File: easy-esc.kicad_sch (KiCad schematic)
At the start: 43 parts, among them J101 USB_C_Receptacle_USB2.0, J102 BLDC, J103 POWER, SW101 BOOT, SW102 RESET, SW103 EN, U101 TMC6300, U102 XC6206, U103 W25Q128JVS, U104 RP2040, Y101 12MHz

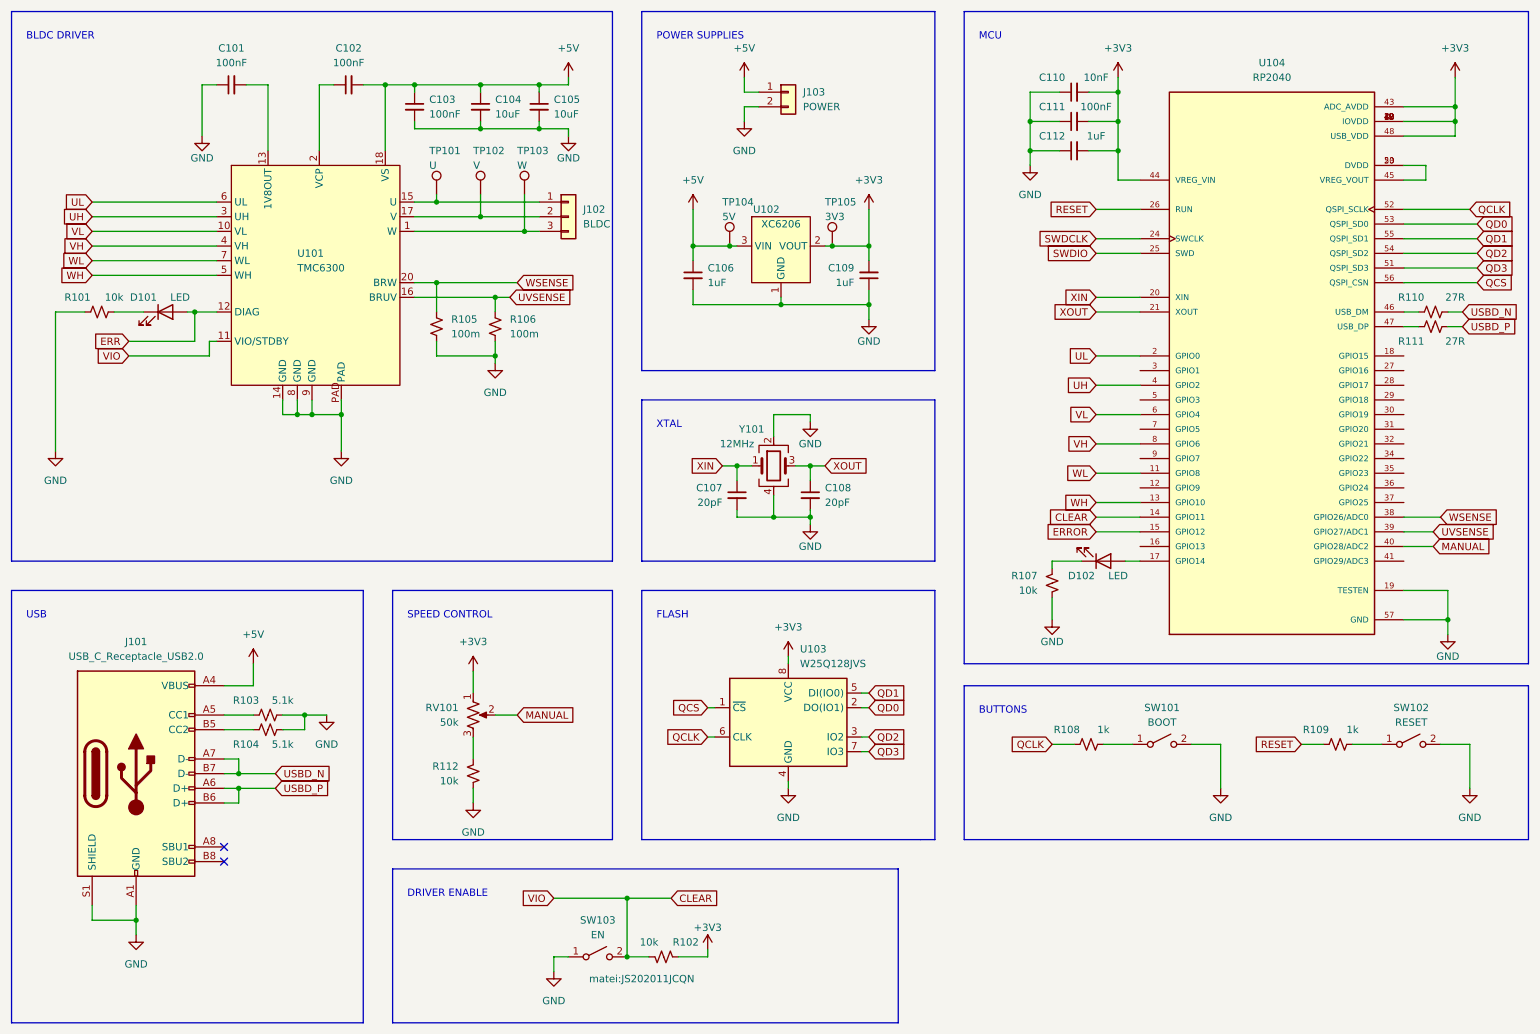
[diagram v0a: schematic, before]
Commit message: finalize fab files
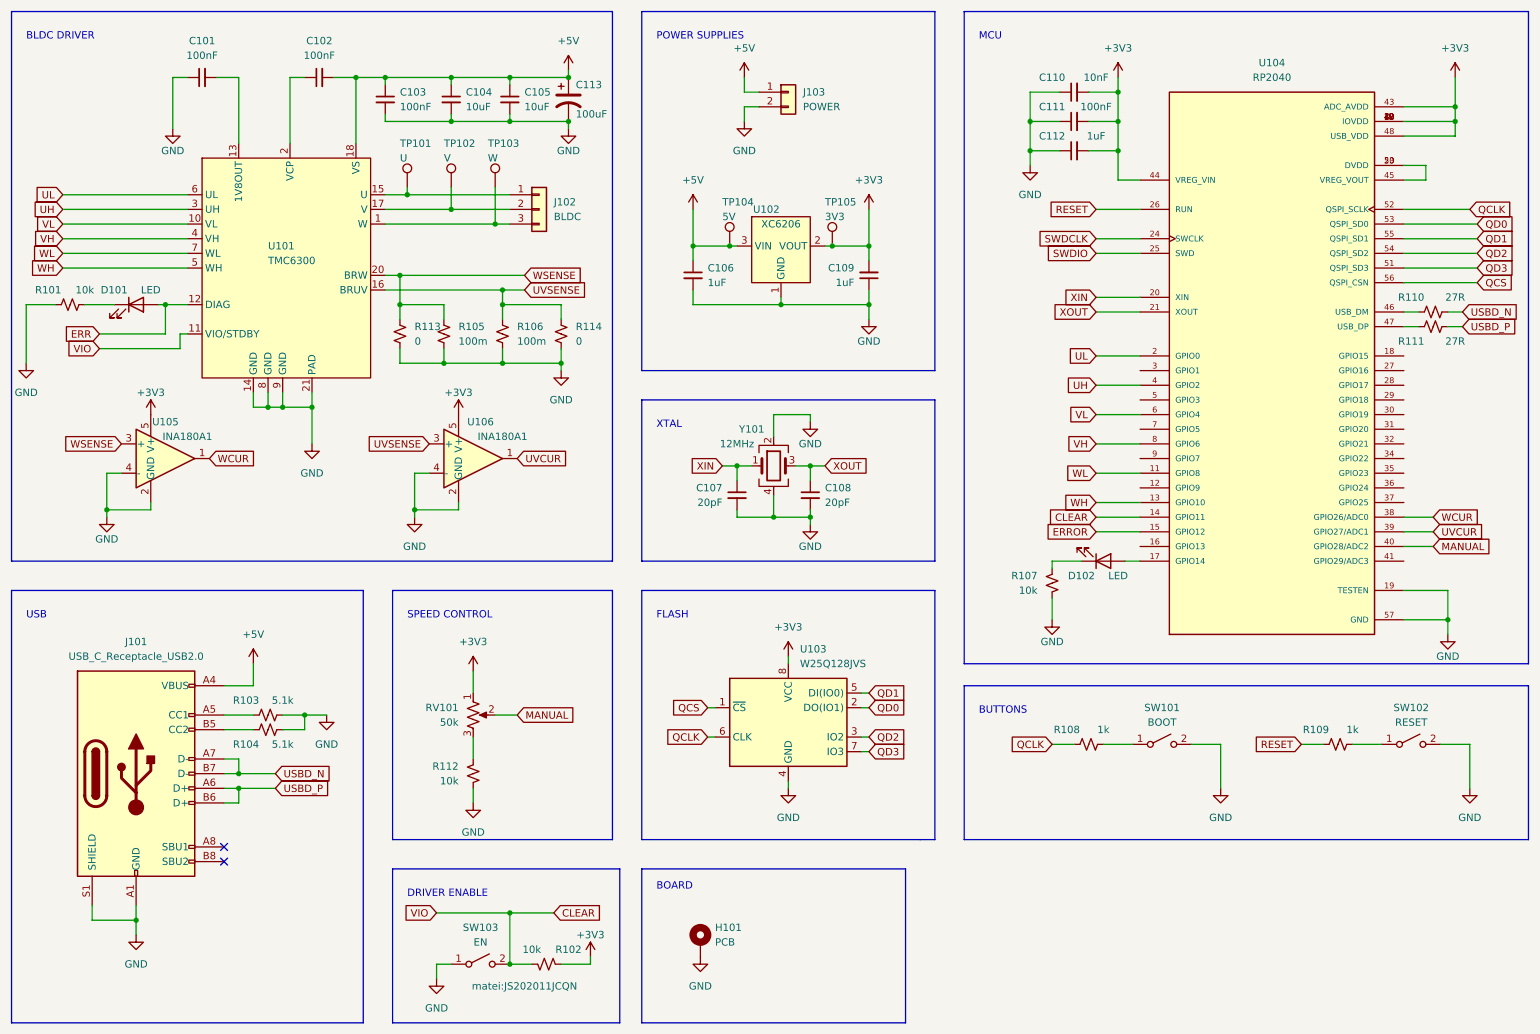
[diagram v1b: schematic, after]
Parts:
- added C113: 100uF, Capacitor_SMD:CP_Elec_4x3.9, symbol Device:C_Polarized_US
- added H101: PCB, matei:easy-esc-outline, symbol Mechanical:MountingHole_Pad
- added R113, R114: 0, Resistor_SMD:R_0402_1005Metric, symbol Device:R_Small_US
- added U105, U106: INA180A1, Package_TO_SOT_SMD:SOT-23-5, symbol Amplifier_Current:INA180A1
- R105, R106: footprint Resistor_SMD:R_0402_1005Metric -> Resistor_SMD:R_2512_6332Metric
- TP101, TP102, TP103, TP104, TP105: footprint TestPoint:TestPoint_Loop_D1.80mm_Drill1.0mm_Beaded -> TestPoint:TestPoint_Pad_D1.5mm
- U101: footprint Package_DFN_QFN:QFN-20-1EP_3x3mm_P0.4mm_EP1.65x1.65mm_ThermalVias -> Package_DFN_QFN:QFN-20-1EP_3x3mm_P0.4mm_EP1.65x1.65mm
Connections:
- net +3V3: now also U105.5 (V+), U106.5 (V+)
- net +5V: now also C113.1
- net GND: now also U101.21 (PAD), C113.2, H101.1, R113.2, R114.2, U105.2 (GND), U105.4 (-), U106.2 (GND), U106.4 (-); no longer U101.PAD
- net UVSENSE: now also R114.1, U106.3 (+); no longer U104.39 (GPIO27/ADC1)
- net WSENSE: now also R113.1, U105.3 (+); no longer U104.38 (GPIO26/ADC0)
- new net UVCUR: U104.39 (GPIO27/ADC1), U106.1
- new net WCUR: U104.38 (GPIO26/ADC0), U105.1
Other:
- note added: "BOARD"
- moved on the sheet: C101, C102, C103, C104, C105, D101, J102, R101, R102, R105, R106, SW103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
